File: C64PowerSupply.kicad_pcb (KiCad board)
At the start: 2 copper layers, 127 x 76.2 mm, 32 parts, among them J1 120V IN, J2 OUT C64, J3 OUT C128, SW1 120/240V SELECT, U1 BD9E303EFJ-LBE2

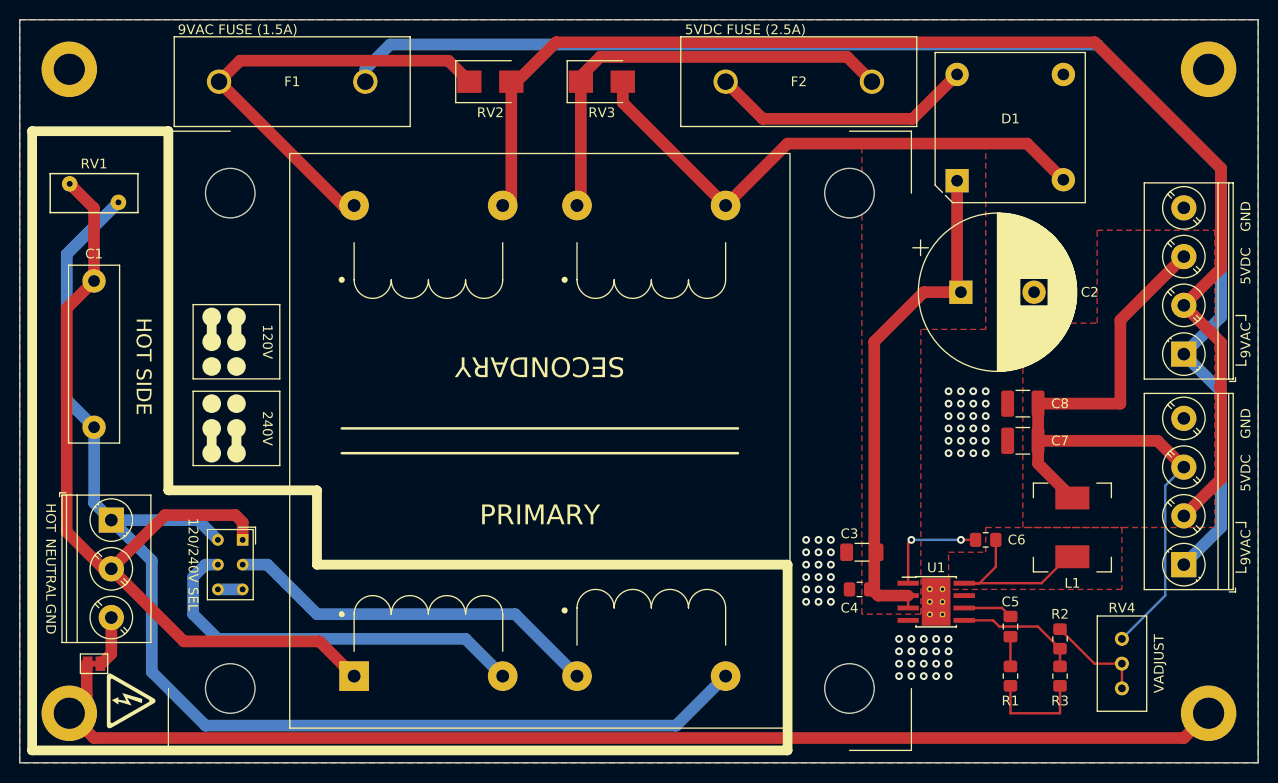
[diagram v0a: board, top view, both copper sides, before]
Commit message: tweak
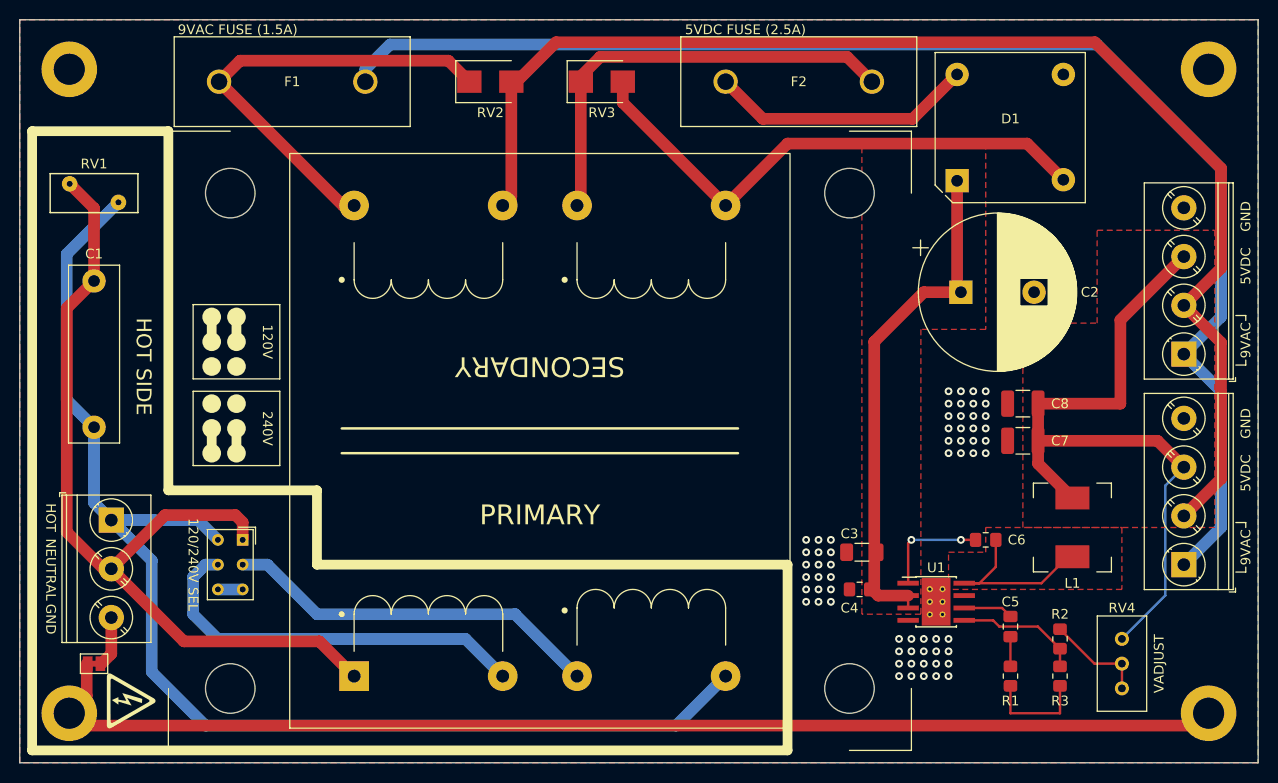
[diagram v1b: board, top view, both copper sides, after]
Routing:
- net GND: track 135.5 -> 134.4 mm
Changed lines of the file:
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@@
       (sketchpadsonfab false)
       (subtractmaskfromsilk true)
-      (outputformat 1)
+      (outputformat 5)
       (mirror false)
       (drillshape 0)
       (scaleselection 1)
-      (outputdirectory "plot")
+      (outputdirectory "img")
     )
   )
@@
     (fp_line (start 1.6 1.25) (end -1.6 1.25) (layer "F.Fab") (width 0.1))
     (fp_line (start 1.6 -1.25) (end 1.6 1.25) (layer "F.Fab") (width 0.1))
-    (pad "1" smd roundrect (at -1.5625 0 180) (size 1.325 2.7) (layers "F.Cu" "F.Paste" "F.Mask") (roundrect_rratio 0.188679)
+    (pad "1" smd roundrect (at -1.5625 0 180) (size 1.325 2.7) (layers "F.Cu" "F.Paste" "F.Mask") (roundrect_rratio 0.1886792453)
       (net 11 "5VDC") (pintype "passive"))
-    (pad "2" smd roundrect (at 1.5625 0 180) (size 1.325 2.7) (layers "F.Cu" "F.Paste" "F.Mask") (roundrect_rratio 0.188679)
+    (pad "2" smd roundrect (at 1.5625 0 180) (size 1.325 2.7) (layers "F.Cu" "F.Paste" "F.Mask") (roundrect_rratio 0.1886792453)
       (net 3 "GND") (pintype "passive"))
     (model "${KICAD6_3DMODEL_DIR}/Capacitor_SMD.3dshapes/C_1210_3225Metric.wrl"
@@
     (fp_line (start 1 0.625) (end -1 0.625) (layer "F.Fab") (width 0.1))
     (fp_line (start -1 -0.625) (end 1 -0.625) (layer "F.Fab") (width 0.1))
-    (pad "1" smd roundrect (at -1 0 270) (size 1.2 1.4) (layers "F.Cu" "F.Paste" "F.Mask") (roundrect_rratio 0.208333)
+    (pad "1" smd roundrect (at -1 0 270) (size 1.2 1.4) (layers "F.Cu" "F.Paste" "F.Mask") (roundrect_rratio 0.2083333333)
       (net 12 "/FB") (pintype "passive"))
-    (pad "2" smd roundrect (at 1 0 270) (size 1.2 1.4) (layers "F.Cu" "F.Paste" "F.Mask") (roundrect_rratio 0.208333)
+    (pad "2" smd roundrect (at 1 0 270) (size 1.2 1.4) (layers "F.Cu" "F.Paste" "F.Mask") (roundrect_rratio 0.2083333333)
       (net 3 "GND") (pintype "passive"))
     (model "${KICAD6_3DMODEL_DIR}/Resistor_SMD.3dshapes/R_0805_2012Metric.wrl"
@@
     (fp_line (start -1 -0.625) (end 1 -0.625) (layer "F.Fab") (width 0.1))
     (fp_line (start -1 0.625) (end -1 -0.625) (layer "F.Fab") (width 0.1))
-    (pad "1" smd roundrect (at -1 0 270) (size 1.2 1.4) (layers "F.Cu" "F.Paste" "F.Mask") (roundrect_rratio 0.208333)
+    (pad "1" smd roundrect (at -1 0 270) (size 1.2 1.4) (layers "F.Cu" "F.Paste" "F.Mask") (roundrect_rratio 0.2083333333)
       (net 6 "Net-(R2-Pad1)") (pintype "passive"))
-    (pad "2" smd roundrect (at 1 0 270) (size 1.2 1.4) (layers "F.Cu" "F.Paste" "F.Mask") (roundrect_rratio 0.208333)
+    (pad "2" smd roundrect (at 1 0 270) (size 1.2 1.4) (layers "F.Cu" "F.Paste" "F.Mask") (roundrect_rratio 0.2083333333)
       (net 12 "/FB") (pintype "passive"))
     (model "${KICAD6_3DMODEL_DIR}/Resistor_SMD.3dshapes/R_0805_2012Metric.wrl"
@@
     (fp_line (start 1.6 -0.8) (end 1.6 0.8) (layer "F.Fab") (width 0.1))
     (fp_line (start -1.6 0.8) (end -1.6 -0.8) (layer "F.Fab") (width 0.1))
-    (pad "1" smd roundrect (at -1.5625 0 180) (size 1.325 1.8) (layers "F.Cu" "F.Paste" "F.Mask") (roundrect_rratio 0.188679)
+    (pad "1" smd roundrect (at -1.5625 0 180) (size 1.325 1.8) (layers "F.Cu" "F.Paste" "F.Mask") (roundrect_rratio 0.1886792453)
       (net 4 "/VUNREG") (pintype "passive"))
-    (pad "2" smd roundrect (at 1.5625 0 180) (size 1.325 1.8) (layers "F.Cu" "F.Paste" "F.Mask") (roundrect_rratio 0.188679)
+    (pad "2" smd roundrect (at 1.5625 0 180) (size 1.325 1.8) (layers "F.Cu" "F.Paste" "F.Mask") (roundrect_rratio 0.1886792453)
       (net 3 "GND") (pintype "passive"))
     (model "${KICAD6_3DMODEL_DIR}/Capacitor_SMD.3dshapes/C_1206_3216Metric.wrl"
@@
     (fp_line (start 1 -0.625) (end 1 0.625) (layer "F.Fab") (width 0.1))
     (fp_line (start 1 0.625) (end -1 0.625) (layer "F.Fab") (width 0.1))
-    (pad "1" smd roundrect (at -1.0375 0 90) (size 1.175 1.45) (layers "F.Cu" "F.Paste" "F.Mask") (roundrect_rratio 0.212766)
+    (pad "1" smd roundrect (at -1.0375 0 90) (size 1.175 1.45) (layers "F.Cu" "F.Paste" "F.Mask") (roundrect_rratio 0.2127659574)
       (net 17 "Net-(C5-Pad1)") (pintype "passive"))
-    (pad "2" smd roundrect (at 1.0375 0 90) (size 1.175 1.45) (layers "F.Cu" "F.Paste" "F.Mask") (roundrect_rratio 0.212766)
+    (pad "2" smd roundrect (at 1.0375 0 90) (size 1.175 1.45) (layers "F.Cu" "F.Paste" "F.Mask") (roundrect_rratio 0.2127659574)
       (net 15 "/COMP") (pintype "passive"))
     (model "${KICAD6_3DMODEL_DIR}/Capacitor_SMD.3dshapes/C_0805_2012Metric.wrl"
@@
     (fp_line (start 1 0.625) (end -1 0.625) (layer "F.Fab") (width 0.1))
     (fp_line (start -1 -0.625) (end 1 -0.625) (layer "F.Fab") (width 0.1))
-    (pad "1" smd roundrect (at -1.0375 0) (size 1.175 1.45) (layers "F.Cu" "F.Paste" "F.Mask") (roundrect_rratio 0.212766)
+    (pad "1" smd roundrect (at -1.0375 0) (size 1.175 1.45) (layers "F.Cu" "F.Paste" "F.Mask") (roundrect_rratio 0.2127659574)
       (net 16 "/BOOT") (pintype "passive"))
-    (pad "2" smd roundrect (at 1.0375 0) (size 1.175 1.45) (layers "F.Cu" "F.Paste" "F.Mask") (roundrect_rratio 0.212766)
+    (pad "2" smd roundrect (at 1.0375 0) (size 1.175 1.45) (layers "F.Cu" "F.Paste" "F.Mask") (roundrect_rratio 0.2127659574)
       (net 10 "/REG-SW") (pintype "passive"))
     (model "${KICAD6_3DMODEL_DIR}/Capacitor_SMD.3dshapes/C_0805_2012Metric.wrl"
@@
     (fp_line (start 1.6 -1.25) (end 1.6 1.25) (layer "F.Fab") (width 0.1))
     (fp_line (start -1.6 1.25) (end -1.6 -1.25) (layer "F.Fab") (width 0.1))
-    (pad "1" smd roundrect (at -1.5625 0 180) (size 1.325 2.7) (layers "F.Cu" "F.Paste" "F.Mask") (roundrect_rratio 0.188679)
+    (pad "1" smd roundrect (at -1.5625 0 180) (size 1.325 2.7) (layers "F.Cu" "F.Paste" "F.Mask") (roundrect_rratio 0.1886792453)
       (net 11 "5VDC") (pintype "passive"))
-    (pad "2" smd roundrect (at 1.5625 0 180) (size 1.325 2.7) (layers "F.Cu" "F.Paste" "F.Mask") (roundrect_rratio 0.188679)
+    (pad "2" smd roundrect (at 1.5625 0 180) (size 1.325 2.7) (layers "F.Cu" "F.Paste" "F.Mask") (roundrect_rratio 0.1886792453)
       (net 3 "GND") (pintype "passive"))
     (model "${KICAD6_3DMODEL_DIR}/Capacitor_SMD.3dshapes/C_1210_3225Metric.wrl"
@@
     (fp_line (start 1 -0.625) (end 1 0.625) (layer "F.Fab") (width 0.1))
     (fp_line (start -1 0.625) (end -1 -0.625) (layer "F.Fab") (width 0.1))
-    (pad "1" smd roundrect (at -1.0375 0 180) (size 1.175 1.45) (layers "F.Cu" "F.Paste" "F.Mask") (roundrect_rratio 0.212766)
+    (pad "1" smd roundrect (at -1.0375 0 180) (size 1.175 1.45) (layers "F.Cu" "F.Paste" "F.Mask") (roundrect_rratio 0.2127659574)
       (net 4 "/VUNREG") (pintype "passive"))
-    (pad "2" smd roundrect (at 1.0375 0 180) (size 1.175 1.45) (layers "F.Cu" "F.Paste" "F.Mask") (roundrect_rratio 0.212766)
+    (pad "2" smd roundrect (at 1.0375 0 180) (size 1.175 1.45) (layers "F.Cu" "F.Paste" "F.Mask") (roundrect_rratio 0.2127659574)
       (net 3 "GND") (pintype "passive"))
     (model "${KICAD6_3DMODEL_DIR}/Capacitor_SMD.3dshapes/C_0805_2012Metric.wrl"
@@
     (fp_line (start -1 0.625) (end -1 -0.625) (layer "F.Fab") (width 0.1))
     (fp_line (start 1 -0.625) (end 1 0.625) (layer "F.Fab") (width 0.1))
-    (pad "1" smd roundrect (at -1 0 270) (size 1.2 1.4) (layers "F.Cu" "F.Paste" "F.Mask") (roundrect_rratio 0.208333)
+    (pad "1" smd roundrect (at -1 0 270) (size 1.2 1.4) (layers "F.Cu" "F.Paste" "F.Mask") (roundrect_rratio 0.2083333333)
       (net 17 "Net-(C5-Pad1)") (pintype "passive"))
-    (pad "2" smd roundrect (at 1 0 270) (size 1.2 1.4) (layers "F.Cu" "F.Paste" "F.Mask") (roundrect_rratio 0.208333)
+    (pad "2" smd roundrect (at 1 0 270) (size 1.2 1.4) (layers "F.Cu" "F.Paste" "F.Mask") (roundrect_rratio 0.2083333333)
       (net 3 "GND") (pintype "passive"))
     (model "${KICAD6_3DMODEL_DIR}/Resistor_SMD.3dshapes/R_0805_2012Metric.wrl"
@@
   (segment (start 76.2 77.59) (end 76.2 70.13) (width 1.2) (layer "F.Cu") (net 2))
   (segment (start 91.44 102.34) (end 90.7 101.6) (width 1.2) (layer "F.Cu") (net 2))
-  (segment (start 76.2 124.46) (end 187.96 124.46) (width 1.2) (layer "F.Cu") (net 3))
+  (segment (start 189.23 123.19) (end 190.5 121.92) (width 1.2) (layer "F.Cu") (net 3))
+  (segment (start 73.66 121.92) (end 74.93 123.19) (width 1.2) (layer "F.Cu") (net 3))
   (segment (start 73.66 121.92) (end 75.45 120.13) (width 1.2) (layer "F.Cu") (net 3))
   (segment (start 170.18 121.92) (end 175.26 121.92) (width 0.25) (layer "F.Cu") (net 3))
   (segment (start 170.18 119.11) (end 170.18 121.92) (width 0.25) (layer "F.Cu") (net 3))
-  (segment (start 73.66 121.92) (end 76.2 124.46) (width 1.2) (layer "F.Cu") (net 3))
   (segment (start 75.45 120.13) (end 75.45 116.84) (width 1.2) (layer "F.Cu") (net 3))
+  (segment (start 74.93 123.19) (end 189.23 123.19) (width 1.2) (layer "F.Cu") (net 3))
   (segment (start 175.26 121.92) (end 175.26 119.11) (width 0.25) (layer "F.Cu") (net 3))
-  (segment (start 187.96 124.46) (end 190.5 121.92) (width 1.2) (layer "F.Cu") (net 3))
   (via (at 163.83 95.25) (size 0.8) (drill 0.4) (layers "F.Cu" "B.Cu") (free) (net 3))
   (via (at 163.83 115.57) (size 0.8) (drill 0.4) (layers "F.Cu" "B.Cu") (free) (net 3))
